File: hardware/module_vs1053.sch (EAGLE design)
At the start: 118 parts, among them IC1 IC_USBLC6-2, IC2 LM1117IMPX-3.3, IC3 PIC32MX795F512, IC4 DP83848, IC5 LM1117MPX-2.5, J1 AUDIO_JACK_TRRSSMD_RA, U1 USD-SOCKETUSD, U3 VS1053-L, X2 CRYSTALS-NOGND-CFPX-217, X3 KUSBVX, Y3 CRYSTAL-GROUNDEDSMD-5X3.2

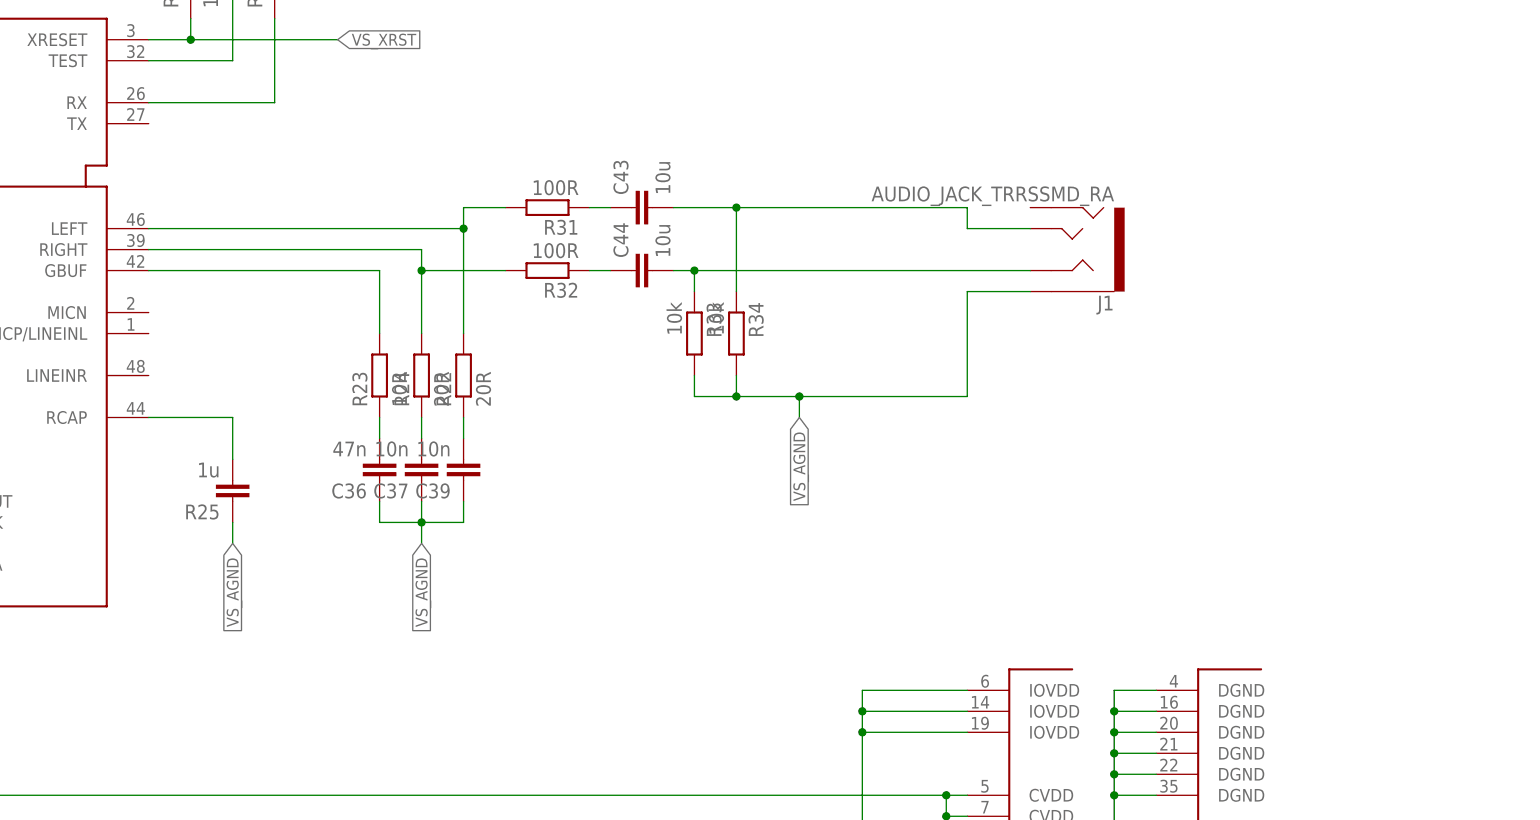
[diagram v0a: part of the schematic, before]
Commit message: ADC (work in progress)
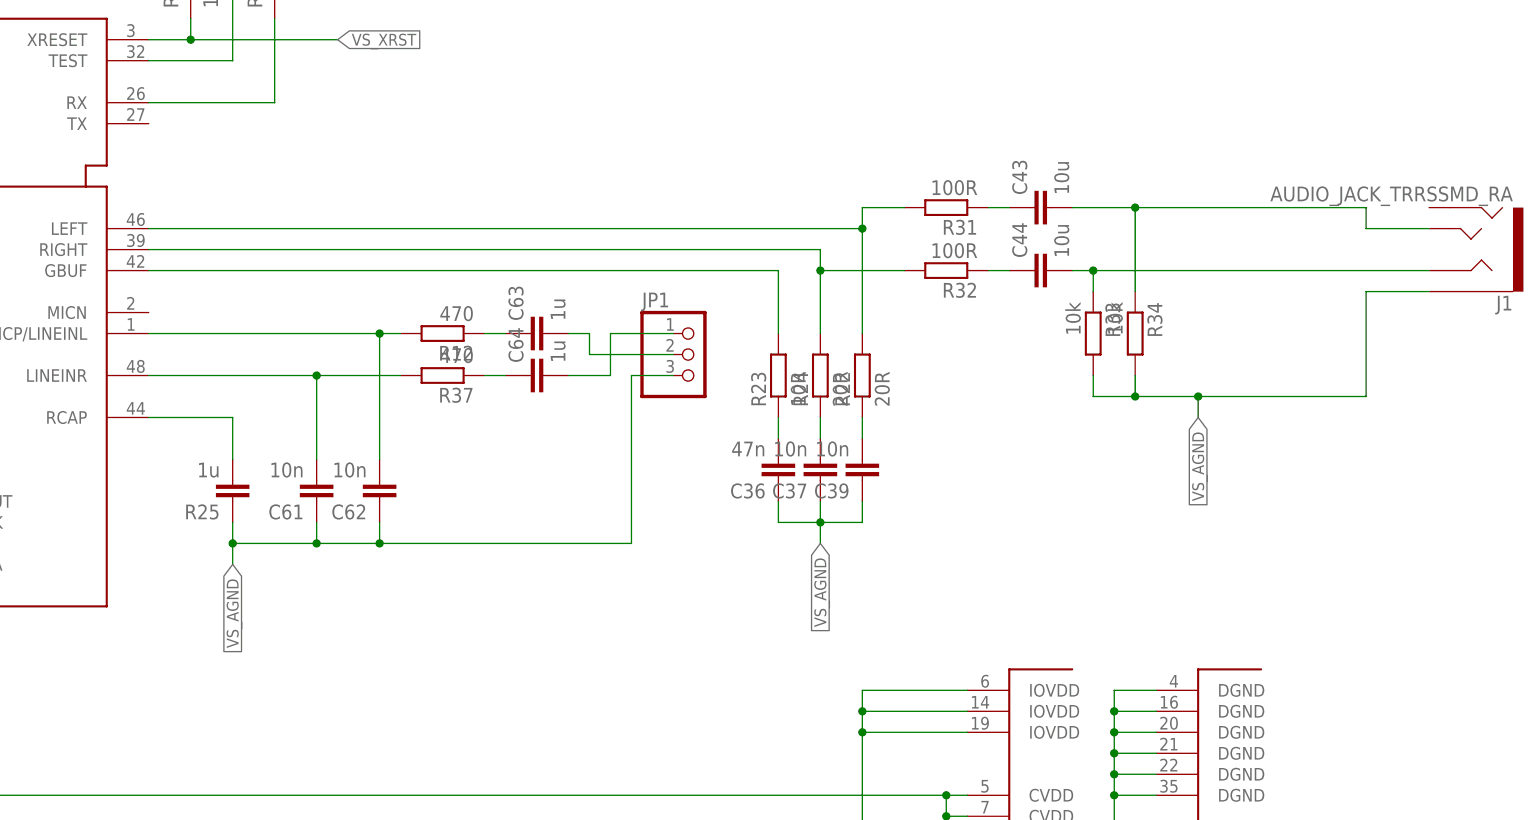
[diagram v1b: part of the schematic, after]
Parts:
- added C61, C62: 10n, rcl:C-EUC0603
- added C63, C64: 1u, rcl:C-EUC0603
- added JP1: (no value), pinhead:PINHD-1X3
- added R12, R37: 470, rcl:R-EU_0204/5
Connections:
- new net IN_LEFT: C63.2, JP1.2
- new net IN_RIGHT: C64.2, JP1.1
- new net N$13: C62.2, R12.2, U3G$1.MICP/LINEINL
- new net N$14: C64.1, R37.1
- new net N$15: C63.1, R12.1
- new net N$5: C61.2, R37.2, U3G$1.LINEINR
- net VS_AGND: now also C61.1, C62.1, JP1.3
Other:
- moved on the sheet: C36, C37, C39, C43, C44, J1, R22, R23, R24, R31, R32, R33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
